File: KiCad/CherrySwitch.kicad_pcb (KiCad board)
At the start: 2 copper layers, 35.6 x 30 mm, 2 parts, among them J1 AudioJack_Mono_Ground_Switch, SW1 SW_Push

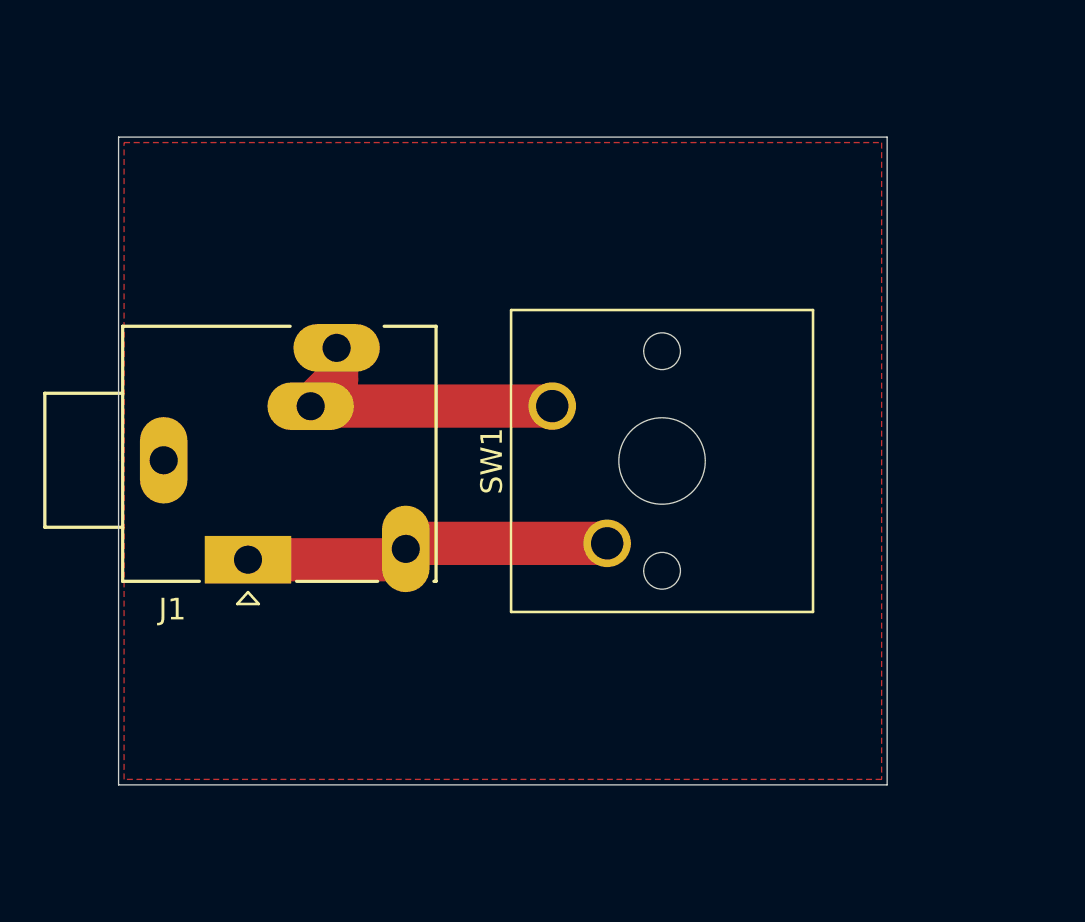
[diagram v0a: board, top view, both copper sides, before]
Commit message: updates
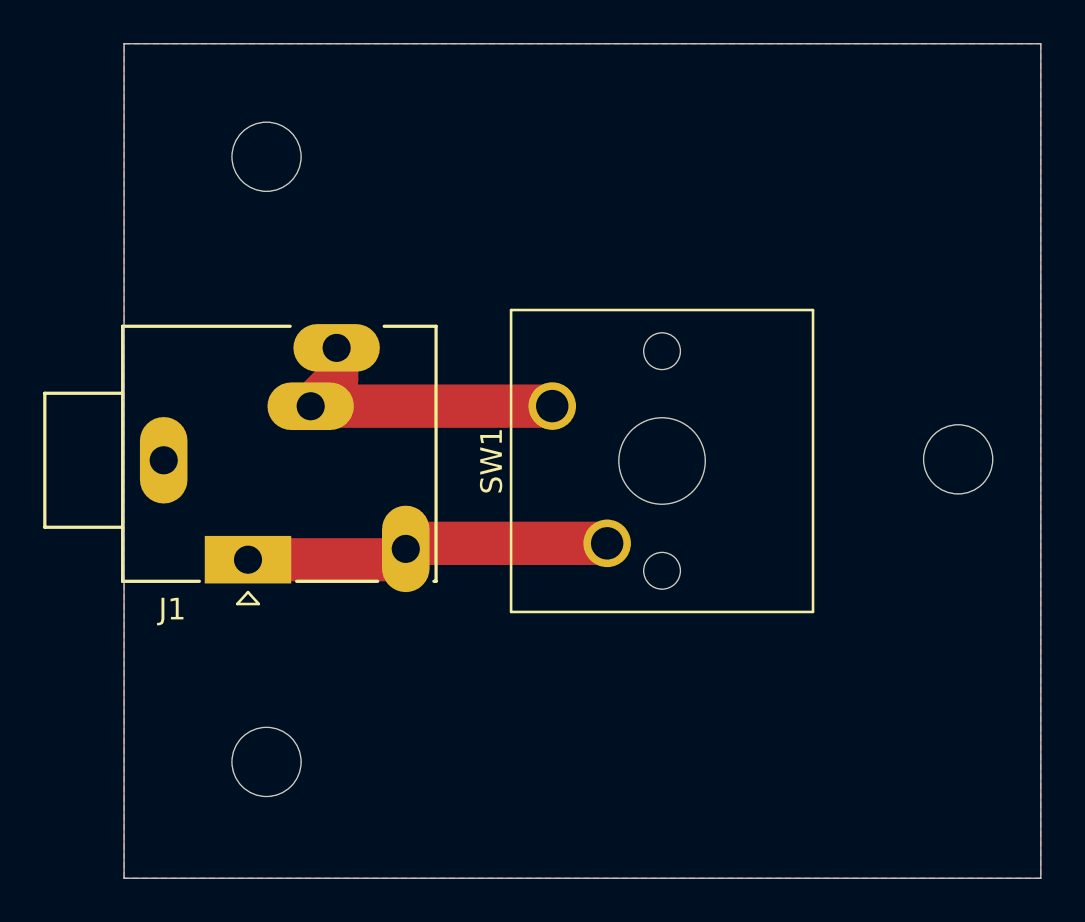
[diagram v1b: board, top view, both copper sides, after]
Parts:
- added ?: 3.2mm_M3, MountingHole:MountingHole_3.2mm_M3, F.Cu at (159.8, 68.2)
- added ?: , MountingHole:MountingHole_3.2mm_M3, F.Cu at (127.8, 54.2)
- added ?: , MountingHole:MountingHole_3.2mm_M3, F.Cu at (127.8, 82.2)
- added ?: MX_Stabilizer_Cutout-2u, Keebio-Parts:MX_Stabilizer_Cutout-2u, F.Cu at (146.1, 68.3)
- J1: value AudioJack_Mono_Ground_Switch -> Jack_Mono
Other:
- board size 35.6 x 30 mm -> 42.4 x 38.6 mm
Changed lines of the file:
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@@
-(kicad_pcb (version 20171130) (host pcbnew "(6.0.0-rc1-dev-1521-g81a0ab4d7)")
+(kicad_pcb (version 20171130) (host pcbnew "(5.0.2)-1")
   (general
     (thickness 1.6)
-    (drawings 5)
+    (drawings 4)
     (tracks 6)
     (zones 0)
-    (modules 2)
+    (modules 6)
     (nets 4)
   )
@@
   )
   (setup
-    (last_trace_width 2)
+    (last_trace_width 0.25)
     (user_trace_width 2)
     (trace_clearance 0.254)
@@
     (zone_45_only no)
     (trace_min 0.127)
+    (segment_width 0.2)
+    (edge_width 0.05)
     (via_size 0.6858)
     (via_drill 0.3302)
@@
     (uvia_min_size 0)
     (uvia_min_drill 0)
-    (edge_width 0.05)
-    (segment_width 0.2)
     (pcb_text_width 0.3)
     (pcb_text_size 1.5 1.5)
@@
     (solder_mask_min_width 0.25)
     (aux_axis_origin 0 0)
-    (visible_elements FFFFFF7F)
+    (visible_elements 7FFFFFFF)
     (pcbplotparams
-      (layerselection 0x010fc_ffffffff)
-      (usegerberextensions false)
+      (layerselection 0x010f0_ffffffff)
+      (usegerberextensions true)
       (usegerberattributes false)
       (usegerberadvancedattributes false)
@@
       (outputformat 1)
       (mirror false)
-      (drillshape 1)
+      (drillshape 0)
       (scaleselection 1)
-      (outputdirectory ""))
+      (outputdirectory "../Gerbers/"))
   )
   (net 0 "")
@@
     (add_net "Net-(J1-PadT)")
   )
+  (module MountingHole:MountingHole_3.2mm_M3 (layer F.Cu)
+    (at 159.75 68.25)
+    (descr "Mounting Hole 3.2mm, no annular, M3")
+    (tags "mounting hole 3.2mm no annular m3")
+    (attr virtual)
+    (fp_text reference "" (at 0 -4.2) (layer F.SilkS)
+      (effects (font (size 1 1) (thickness 0.15)))
+    )
+    (fp_text value 3.2mm_M3 (at 0.778 7.696 90) (layer F.Fab)
+      (effects (font (size 1 1) (thickness 0.15)))
+    )
+    (fp_text user %R (at 0.3 0) (layer F.Fab)
+      (effects (font (size 1 1) (thickness 0.15)))
+    )
+    (fp_circle (center 0 0) (end 3.2 0) (layer Cmts.User) (width 0.15))
+    (fp_circle (center 0 0) (end 3.45 0) (layer F.CrtYd) (width 0.05))
+    (pad 1 np_thru_hole circle (at 0 0) (size 3.2 3.2) (drill 3.2) (layers *.Cu *.Mask))
+  )
   (module Connector_Audio:Jack_3.5mm_Ledino_KB3SPRS_Horizontal (layer F.Cu)
     (at 126.893001 72.893001)
@@
       (effects (font (size 1 1) (thickness 0.15)))
     )
-    (fp_text value AudioJack_Mono_Ground_Switch (at 2.3 -12.2) (layer F.Fab)
+    (fp_text value Jack_Mono (at 2.3 -12.2) (layer F.Fab)
       (effects (font (size 1 1) (thickness 0.15)))
     )
@@
     )
   )
-  (gr_line (start 156.464 53.34) (end 120.904 53.34) (angle 90) (layer Edge.Cuts) (width 0.05))
-  (gr_line (start 156.464 83.312) (end 156.464 53.34) (angle 90) (layer Edge.Cuts) (width 0.05))
-  (gr_line (start 120.904 83.312) (end 156.464 83.312) (angle 90) (layer Edge.Cuts) (width 0.05))
-  (gr_line (start 120.904 68.326) (end 120.904 83.312) (angle 90) (layer Edge.Cuts) (width 0.05))
-  (gr_line (start 120.904 68.326) (end 120.904 53.34) (angle 90) (layer Edge.Cuts) (width 0.05))
+  (module MountingHole:MountingHole_3.2mm_M3 (layer F.Cu)
+    (at 127.75 54.25)
+    (descr "Mounting Hole 3.2mm, no annular, M3")
+    (tags "mounting hole 3.2mm no annular m3")
+    (attr virtual)
+    (fp_text reference "" (at 0 -4.2) (layer F.SilkS)
+      (effects (font (size 1 1) (thickness 0.15)))
+    )
+    (fp_text value "" (at 0 4.2) (layer F.Fab)
+      (effects (font (size 1 1) (thickness 0.15)))
+    )
+    (fp_circle (center 0 0) (end 3.45 0) (layer F.CrtYd) (width 0.05))
+    (fp_circle (center 0 0) (end 3.2 0) (layer Cmts.User) (width 0.15))
+    (fp_text user %R (at 0.3 0) (layer F.Fab)
+      (effects (font (size 1 1) (thickness 0.15)))
+    )
+    (pad 1 np_thru_hole circle (at 0 0) (size 3.2 3.2) (drill 3.2) (layers *.Cu *.Mask))
+  )
+  (module MountingHole:MountingHole_3.2mm_M3 (layer F.Cu)
+    (at 127.75 82.25)
+    (descr "Mounting Hole 3.2mm, no annular, M3")
+    (tags "mounting hole 3.2mm no annular m3")
+    (attr virtual)
+    (fp_text reference "" (at 0 -4.2) (layer F.SilkS)
+      (effects (font (size 1 1) (thickness 0.15)))
+    )
+    (fp_text value "" (at 0 4.2) (layer F.Fab)
+      (effects (font (size 1 1) (thickness 0.15)))
+    )
+    (fp_circle (center 0 0) (end 3.45 0) (layer F.CrtYd) (width 0.05))
+    (fp_circle (center 0 0) (end 3.2 0) (layer Cmts.User) (width 0.15))
+    (fp_text user %R (at 0.3 0) (layer F.Fab)
+      (effects (font (size 1 1) (thickness 0.15)))
+    )
+    (pad 1 np_thru_hole circle (at 0 0) (size 3.2 3.2) (drill 3.2) (layers *.Cu *.Mask))
+  )
+  (module Keebio-Parts:MX_Stabilizer_Cutout-2u (layer F.Cu)
+    (at 146.05 68.326 90)
+    (fp_text reference "" (at 0.25 10.05 90) (layer Eco2.User) hide
+      (effects (font (size 1 1) (thickness 0.15)))
+    )
+    (fp_text value MX_Stabilizer_Cutout-2u (at 17.272 0 180) (layer F.Fab) hide
+      (effects (font (size 1 1) (thickness 0.15)))
+    )
+    (fp_line (start 19 -9.5) (end 19 9.5) (layer Dwgs.User) (width 0.15))
+    (fp_line (start 19 9.5) (end -19 9.5) (layer Dwgs.User) (width 0.15))
+    (fp_line (start -19 9.5) (end -19 -9.5) (layer Dwgs.User) (width 0.15))
+    (fp_line (start -19 -9.5) (end 19 -9.5) (layer Dwgs.User) (width 0.15))
+    (pad "" np_thru_hole oval (at -11.938 7.7724 90) (size 3.048 0.3048) (drill oval 3.048 0.3048) (layers *.Cu *.Mask))
+    (pad "" np_thru_hole oval (at -10.5664 7.112 90) (size 0.3048 1.4732) (drill oval 0.3048 1.4732) (layers *.Cu *.Mask))
+    (pad "" np_thru_hole oval (at -13.3096 7.112 90) (size 0.3048 1.4732) (drill oval 0.3048 1.4732) (layers *.Cu *.Mask))
+    (pad "" np_thru_hole oval (at -15.5448 0.3556 90) (size 1.1684 0.3048) (drill oval 1.1684 0.3048) (layers *.Cu *.Mask))
+    (pad "" np_thru_hole oval (at -11.938 6.4516 90) (size 6.6548 0.3048) (drill oval 6.6548 0.3048) (layers *.Cu *.Mask))
+    (pad "" np_thru_hole oval (at -8.763 0.4572 90) (size 0.3048 12.2936) (drill oval 0.3048 12.2936) (layers *.Cu *.Mask))
+    (pad "" np_thru_hole oval (at -15.113 0.4572 90) (size 0.3048 12.2936) (drill oval 0.3048 12.2936) (layers *.Cu *.Mask))
+    (pad "" np_thru_hole oval (at -15.9766 -0.889 90) (size 0.3048 2.794) (drill oval 0.3048 2.794) (layers *.Cu *.Mask))
+    (pad "" np_thru_hole oval (at -15.5448 -2.1336 90) (size 1.1684 0.3048) (drill oval 1.1684 0.3048) (layers *.Cu *.Mask))
+    (pad "" np_thru_hole oval (at -11.938 -5.5372 90) (size 6.6548 0.3048) (drill oval 6.6548 0.3048) (layers *.Cu *.Mask))
+    (pad "" np_thru_hole oval (at 15.5448 0.3556 90) (size 1.1684 0.3048) (drill oval 1.1684 0.3048) (layers *.Cu *.Mask))
+    (pad "" np_thru_hole oval (at 13.3096 7.112 90) (size 0.3048 1.4732) (drill oval 0.3048 1.4732) (layers *.Cu *.Mask))
+    (pad "" np_thru_hole oval (at 15.5448 -2.1336 90) (size 1.1684 0.3048) (drill oval 1.1684 0.3048) (layers *.Cu *.Mask))
+    (pad "" np_thru_hole oval (at 10.5664 7.112 90) (size 0.3048 1.4732) (drill oval 0.3048 1.4732) (layers *.Cu *.Mask))
+    (pad "" np_thru_hole oval (at 15.9766 -0.889 90) (size 0.3048 2.794) (drill oval 0.3048 2.794) (layers *.Cu *.Mask))
+    (pad "" np_thru_hole oval (at 15.113 0.4572 90) (size 0.3048 12.2936) (drill oval 0.3048 12.2936) (layers *.Cu *.Mask))
+    (pad "" np_thru_hole oval (at 11.938 6.4516 90) (size 6.6548 0.3048) (drill oval 6.6548 0.3048) (layers *.Cu *.Mask))
+    (pad "" np_thru_hole oval (at 8.763 0.4572 90) (size 0.3048 12.2936) (drill oval 0.3048 12.2936) (layers *.Cu *.Mask))
+    (pad "" np_thru_hole oval (at 11.938 -5.5372 90) (size 6.6548 0.3048) (drill oval 6.6548 0.3048) (layers *.Cu *.Mask))
+    (pad "" np_thru_hole oval (at 11.938 7.7724 90) (size 3.048 0.3048) (drill oval 3.048 0.3048) (layers *.Cu *.Mask))
+  )
+  (gr_line (start 121.158 87.63) (end 163.576 87.63) (angle 90) (layer Edge.Cuts) (width 0.05))
+  (gr_line (start 121.158 49.022) (end 121.158 87.63) (angle 90) (layer Edge.Cuts) (width 0.05))
+  (gr_line (start 163.576 49.022) (end 121.158 49.022) (angle 90) (layer Edge.Cuts) (width 0.05))
+  (gr_line (start 163.576 87.63) (end 163.576 49.022) (angle 90) (layer Edge.Cuts) (width 0.05))
   (segment (start 143.51 72.136) (end 134.450002 72.136) (width 2) (layer F.Cu) (net 1) (status C00000))
   (segment (start 134.450002 72.136) (end 133.693001 72.893001) (width 2) (layer F.Cu) (net 1) (status C00000))
@@
     (connect_pads (clearance 0.508))
     (min_thickness 0.254)
-    (fill yes (arc_segments 32) (thermal_gap 0.508) (thermal_bridge_width 0.508))
+    (fill yes (arc_segments 16) (thermal_gap 0.508) (thermal_bridge_width 0.508))
     (polygon
       (pts
-        (xy 156.21 83.058) (xy 121.158 83.058) (xy 121.158 53.594) (xy 156.21 53.594)
+        (xy 121.158 49.022) (xy 163.576 49.022) (xy 163.576 87.63) (xy 121.158 87.63)
       )
     )
